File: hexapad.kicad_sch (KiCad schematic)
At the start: 2 parts, among them U1 MOUDLE-SEEEDUINO-XIAO, U2 PCF8574A

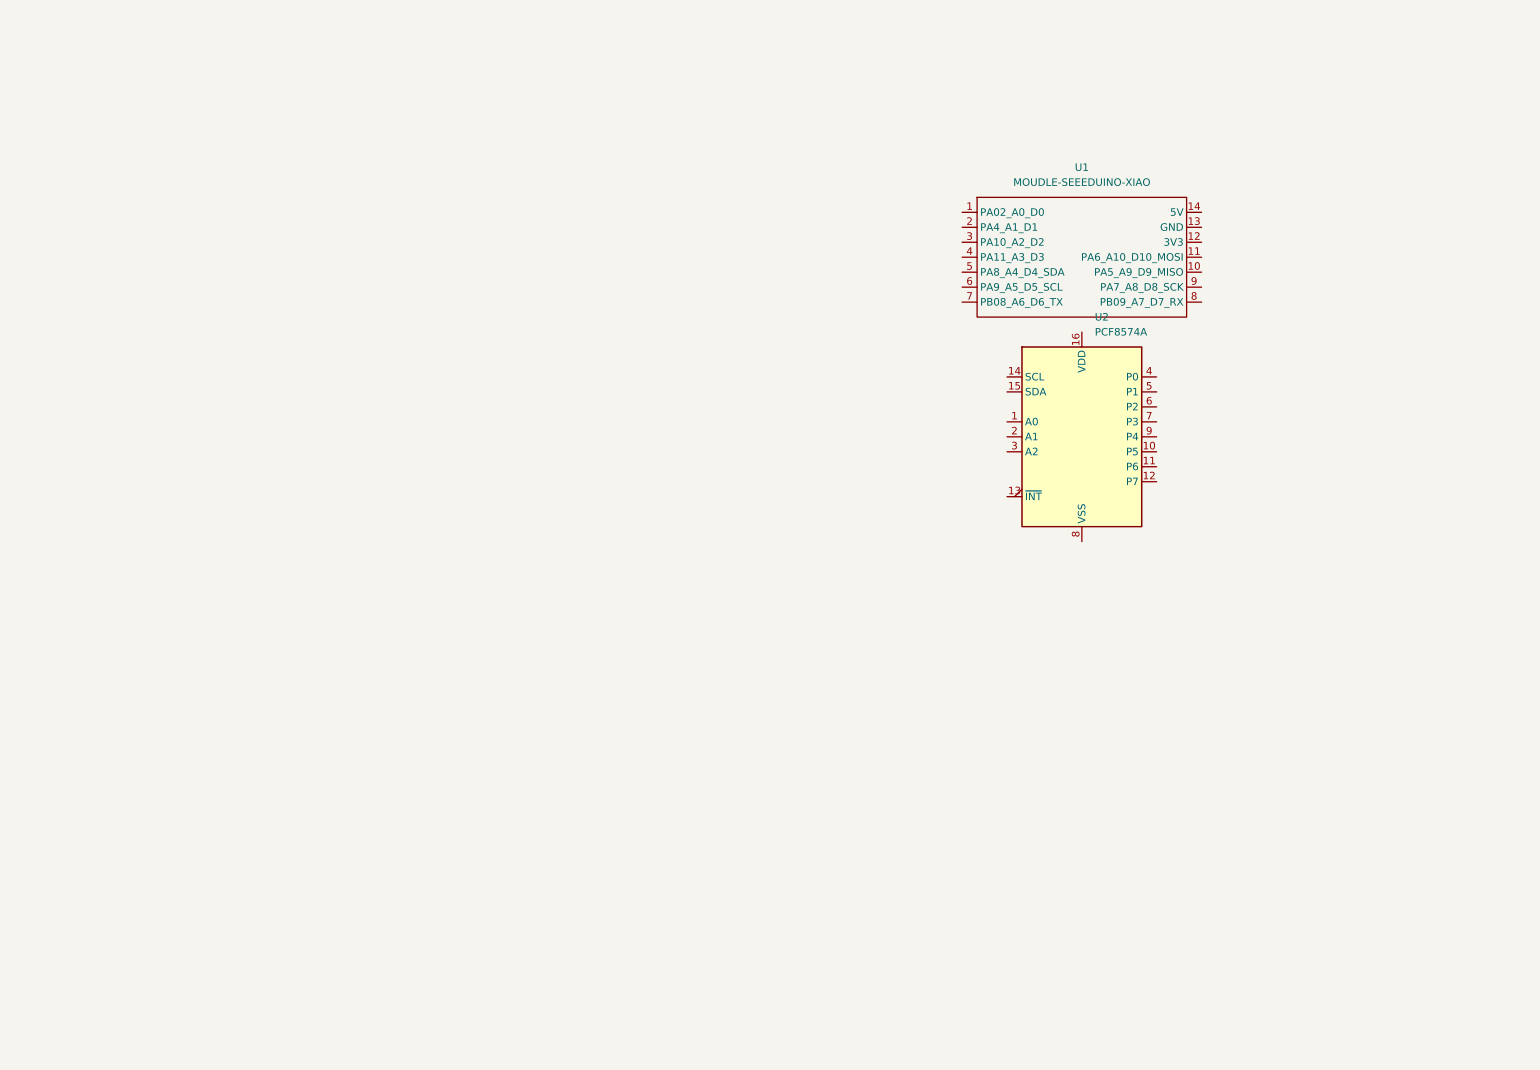
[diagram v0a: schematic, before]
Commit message: a lot lol
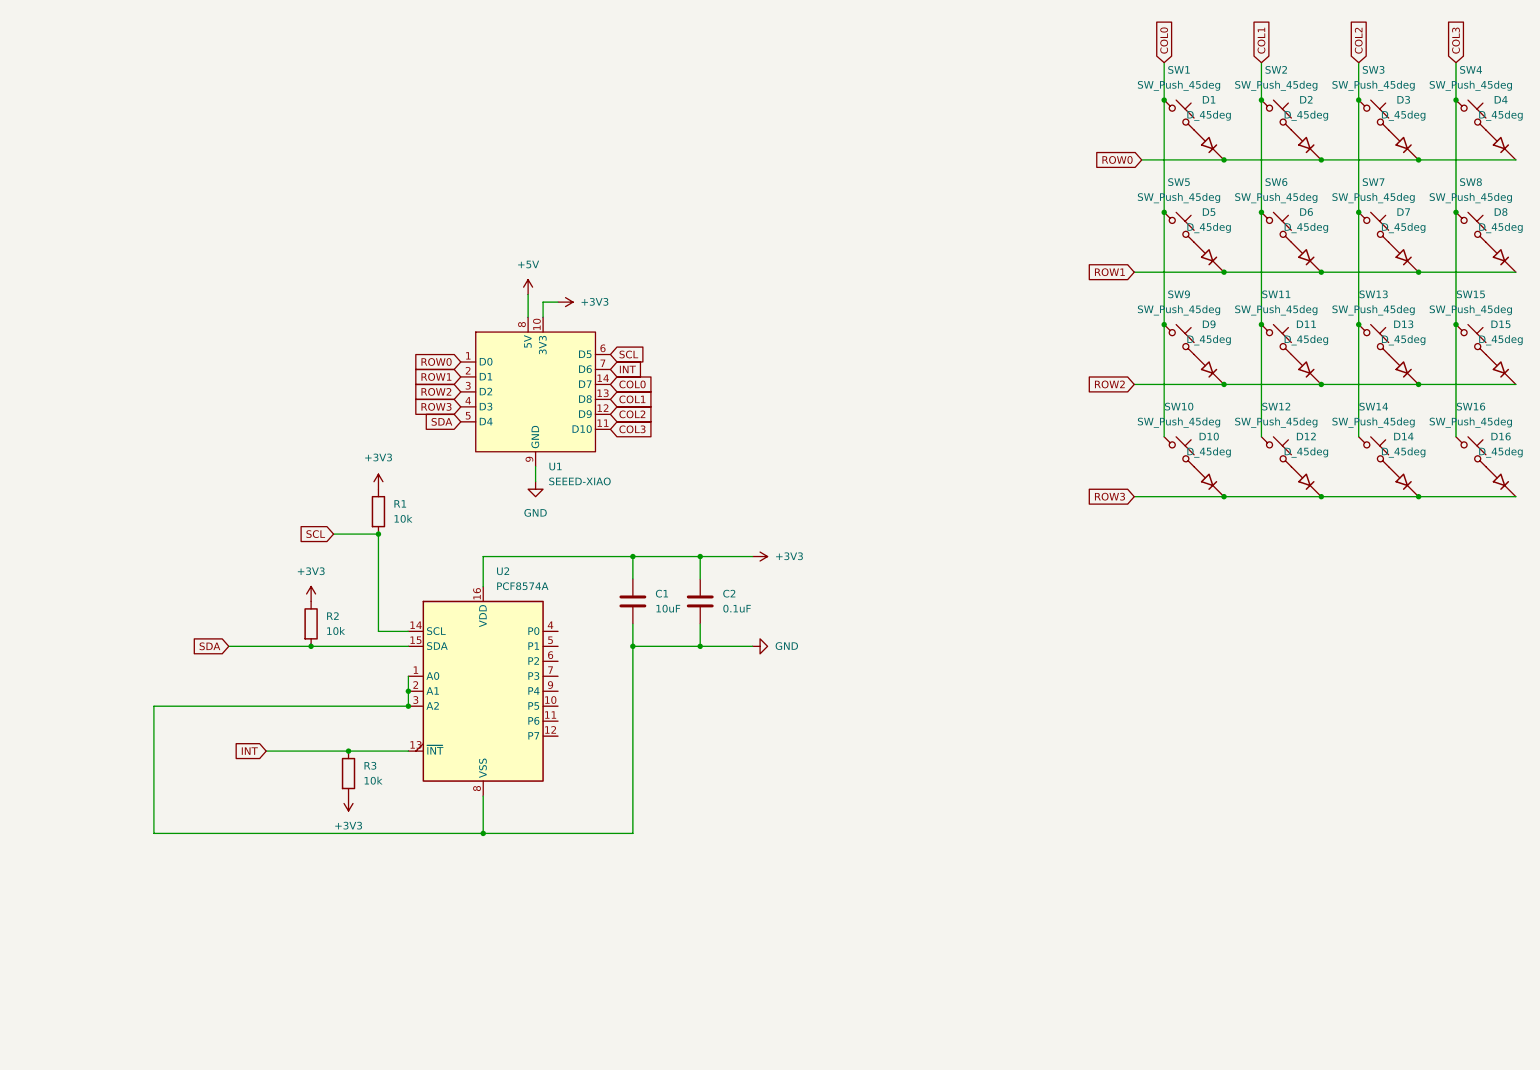
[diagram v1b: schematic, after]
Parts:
- removed U1: MOUDLE-SEEEDUINO-XIAO, symbol MOUDLE-SEEEDUINO-XIAO:MOUDLE-SEEEDUINO-XIAO
- added C1: 10uF, symbol Device:C
- added C2: 0.1uF, symbol Device:C
- added D1, D10, D11, D12, D13, D14, D15, D16, D2, D3, D4, D5, D6, D7, D8, D9: D_45deg, symbol Device:D_45deg
- added R1, R2, R3: 10k, symbol Device:R
- added SW1, SW10, SW11, SW12, SW13, SW14, SW15, SW16, SW2, SW3, SW4, SW5, SW6, SW7, SW8, SW9: SW_Push_45deg, symbol Switch:SW_Push_45deg
- added U1: SEEED-XIAO, XIAO_PCB:XIAO-14P-THT-2.54-21x17.8MM, symbol SEEED-XIAO:SEEED-XIAO
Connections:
- net GND: now reaches U2.1 (A0)
- net GND: now also U2.2 (A1), U2.3 (A2), U2.8 (VSS), C1.2, C2.2, U1.9 (GND)
- net INT: now reaches U2.13 (~{INT})
- net INT: now also R3.1, U1.7 (D6)
- net SCL: now reaches U2.14 (SCL)
- net SCL: now also R1.2, U1.6 (D5)
- net SDA: now reaches U2.15 (SDA)
- net SDA: now also R2.2, U1.5 (D4)
- net +3V3: now reaches U2.16 (VDD)
- net +3V3: now also C1.1, C2.1, R1.1, R2.1, R3.2, U1.10 (3V3)
- new net: D2.2 (A), SW2.2
- new net: D12.2 (A), SW12.2
- new net: D14.2 (A), SW14.2
- new net: D15.2 (A), SW15.2
- new net: D16.2 (A), SW16.2
- new net: D8.2 (A), SW8.2
- new net: D5.2 (A), SW5.2
- new net: D13.2 (A), SW13.2
- new net: D4.2 (A), SW4.2
- new net: D1.2 (A), SW1.2
- new net: D10.2 (A), SW10.2
- new net: D6.2 (A), SW6.2
- new net: D3.2 (A), SW3.2
- new net: D9.2 (A), SW9.2
- new net: D7.2 (A), SW7.2
- new net: D11.2 (A), SW11.2
- new net +5V: U1.8 (5V)
- new net COL0: SW1.1, SW10.1, SW5.1, SW9.1, U1.14 (D7)
- new net COL1: SW11.1, SW12.1, SW2.1, SW6.1, U1.13 (D8)
- new net COL2: SW13.1, SW14.1, SW3.1, SW7.1, U1.12 (D9)
- new net COL3: SW15.1, SW16.1, SW4.1, SW8.1, U1.11 (D10)
- new net ROW0: D1.1 (K), D2.1 (K), D3.1 (K), D4.1 (K), U1.1 (D0)
- new net ROW1: D5.1 (K), D6.1 (K), D7.1 (K), D8.1 (K), U1.2 (D1)
- new net ROW2: D11.1 (K), D13.1 (K), D15.1 (K), D9.1 (K), U1.3 (D2)
- new net ROW3: D10.1 (K), D12.1 (K), D14.1 (K), D16.1 (K), U1.4 (D3)

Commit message: a lot lol, hopefully schematic is done
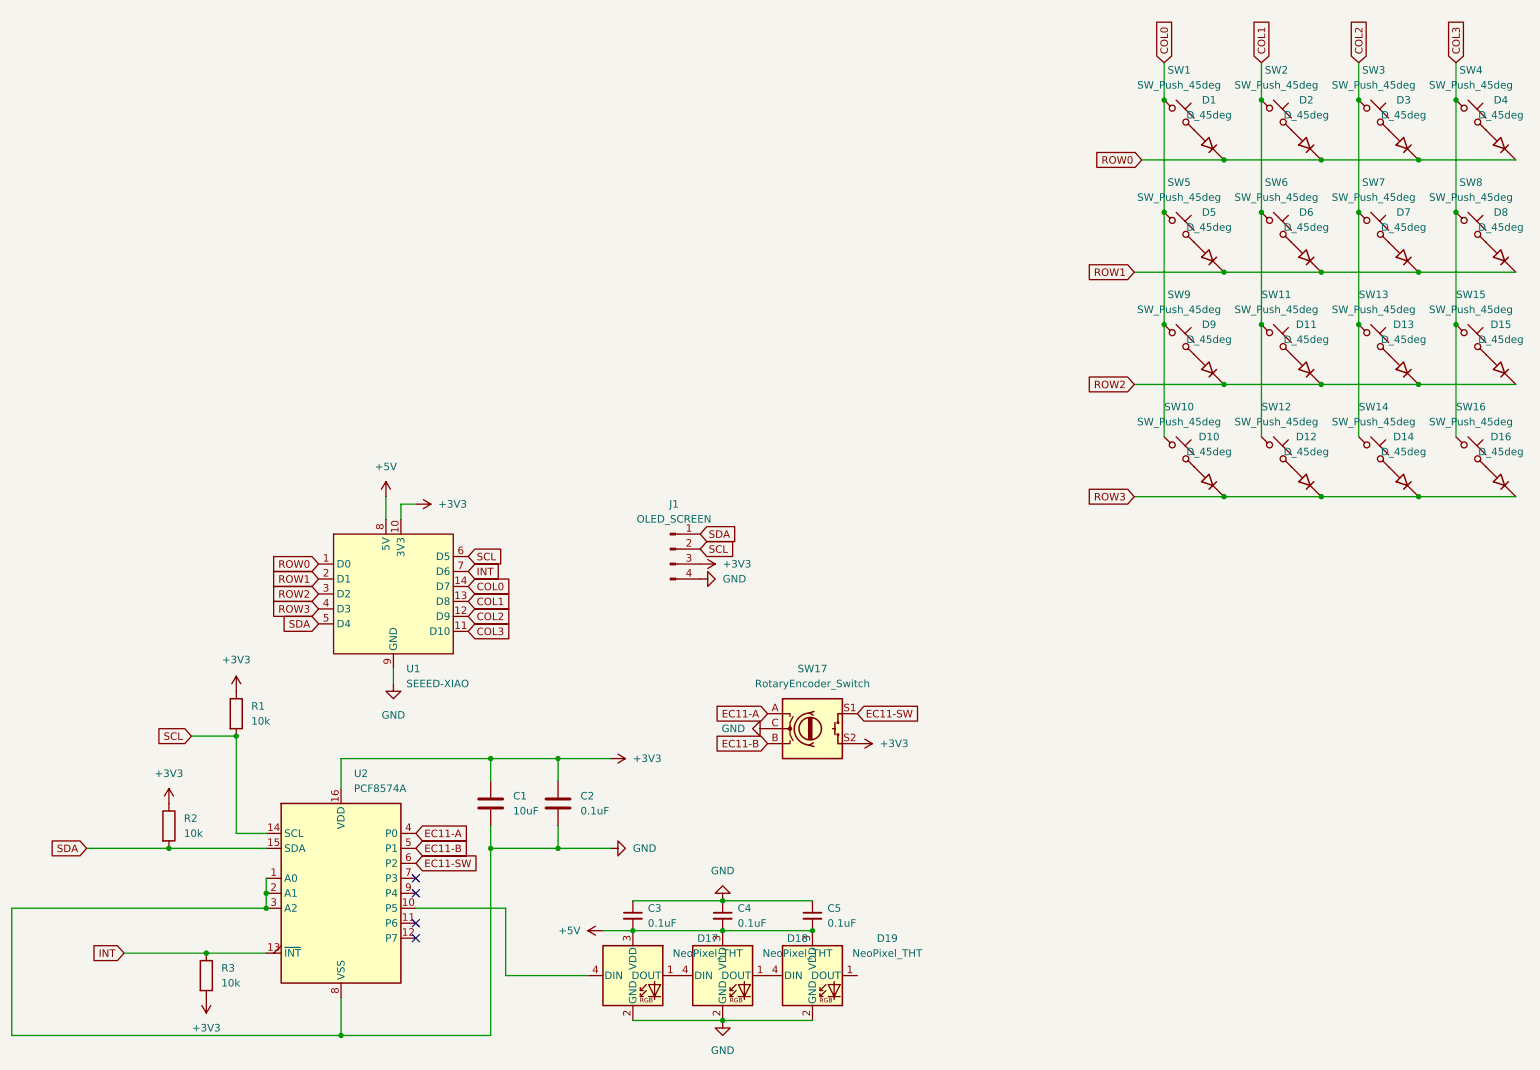
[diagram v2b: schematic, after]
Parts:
- added C3, C4, C5: 0.1uF, symbol Device:C_Small
- added D17, D18, D19: NeoPixel_THT, LED_THT:LED_D5.0mm-4_RGB, symbol LED:NeoPixel_THT
- added J1: OLED_SCREEN, symbol Connector:Conn_01x04_Pin
- added SW17: RotaryEncoder_Switch, symbol Device:RotaryEncoder_Switch
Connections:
- net +3V3: now also J1.3 (Pin_3), SW17.S2
- net +5V: now also C3.2, C4.2, C5.2, D17.3 (VDD), D18.3 (VDD), D19.3 (VDD)
- net GND: now also C3.1, C4.1, C5.1, D17.2 (GND), D18.2 (GND), D19.2 (GND), J1.4 (Pin_4), SW17.C
- net SCL: now also J1.2 (Pin_2)
- net SDA: now also J1.1 (Pin_1)
- net at U2.10 (P5): now also D17.4 (DIN)
- net EC11-A: now reaches U2.4 (P0)
- net EC11-A: now also SW17.A
- net EC11-B: now reaches U2.5 (P1)
- net EC11-B: now also SW17.B
- net EC11-SW: now reaches U2.6 (P2)
- net EC11-SW: now also SW17.S1
- new net: D18.1 (DOUT), D19.4 (DIN)
- new net: D17.1 (DOUT), D18.4 (DIN)
- no-connect marks 0 -> 4
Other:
- moved on the sheet: C1, C2, R1, R2, R3, U1, U2
